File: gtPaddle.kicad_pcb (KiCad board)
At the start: 2 copper layers, 51.4 x 72.6 mm, 36 parts, among them IC1 74157N, IC2 74157N, J1 Conn_01x02_Pin, J2 Conn_01x02_Pin, J3 Conn_01x02_Pin, J4 Conn_01x02_Pin, Q1 2N3904, U1 ADC0804LCN

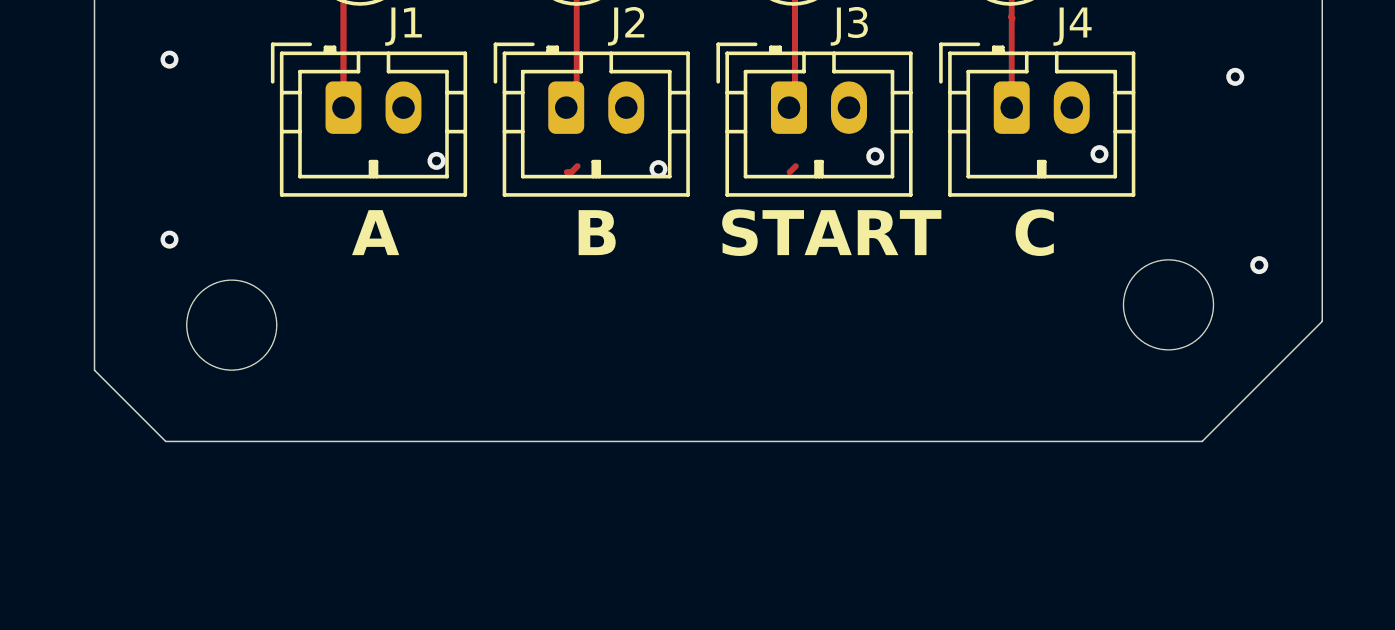
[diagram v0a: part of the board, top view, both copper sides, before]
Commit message: checking edge cuts and mounting points
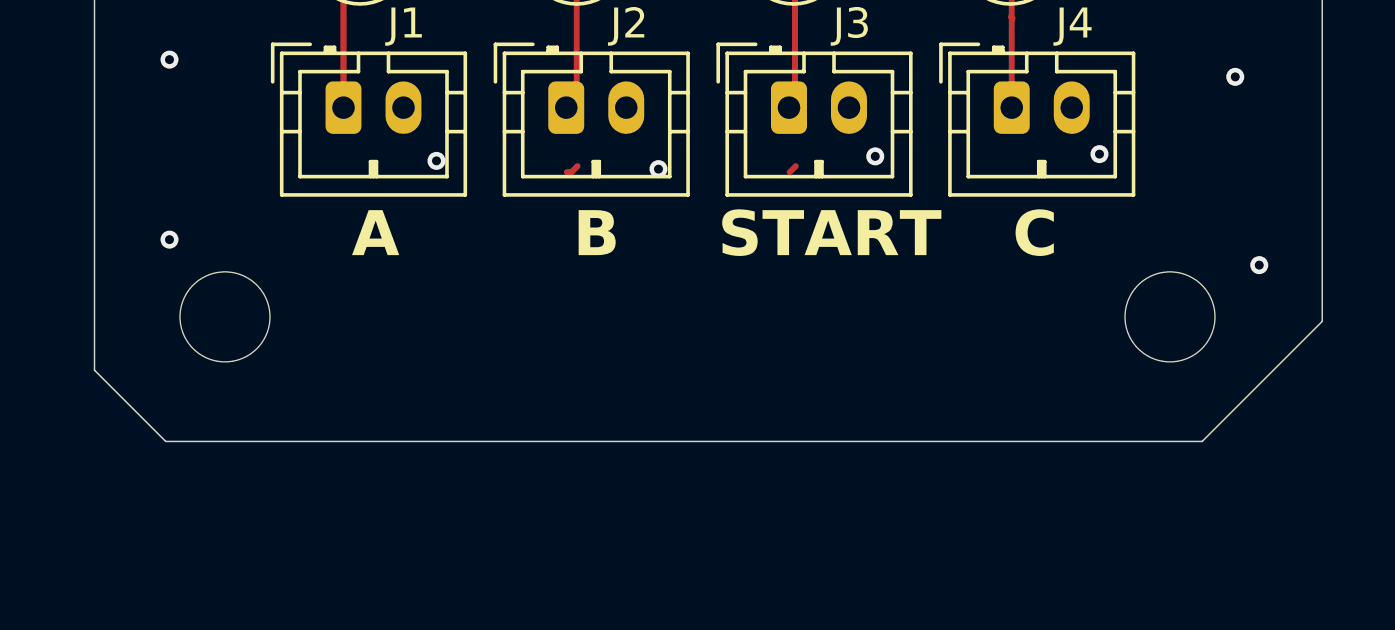
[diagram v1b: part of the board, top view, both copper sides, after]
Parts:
- moved REF** 0.40 mm to (166.5, 136.0)
- moved REF** 0.36 mm to (135.0, 136.0)
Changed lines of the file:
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@@
 	(footprint "MountingHole:MountingHole_3mm"
 		(layer "F.Cu")
-		(at 135.225 136.275)
+		(at 135 136)
 		(descr "Mounting Hole 3mm, no annular, generated by kicad-footprint-generator mountinghole.py")
 		(tags "mountinghole")
@@
 	(footprint "MountingHole:MountingHole_3mm"
 		(layer "F.Cu")
-		(at 166.45 135.6)
+		(at 166.5 136)
 		(descr "Mounting Hole 3mm, no annular, generated by kicad-footprint-generator mountinghole.py")
 		(tags "mountinghole")
